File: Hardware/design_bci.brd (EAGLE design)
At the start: 53.3 x 59.7 mm, 13 parts, among them IC1 AD623N

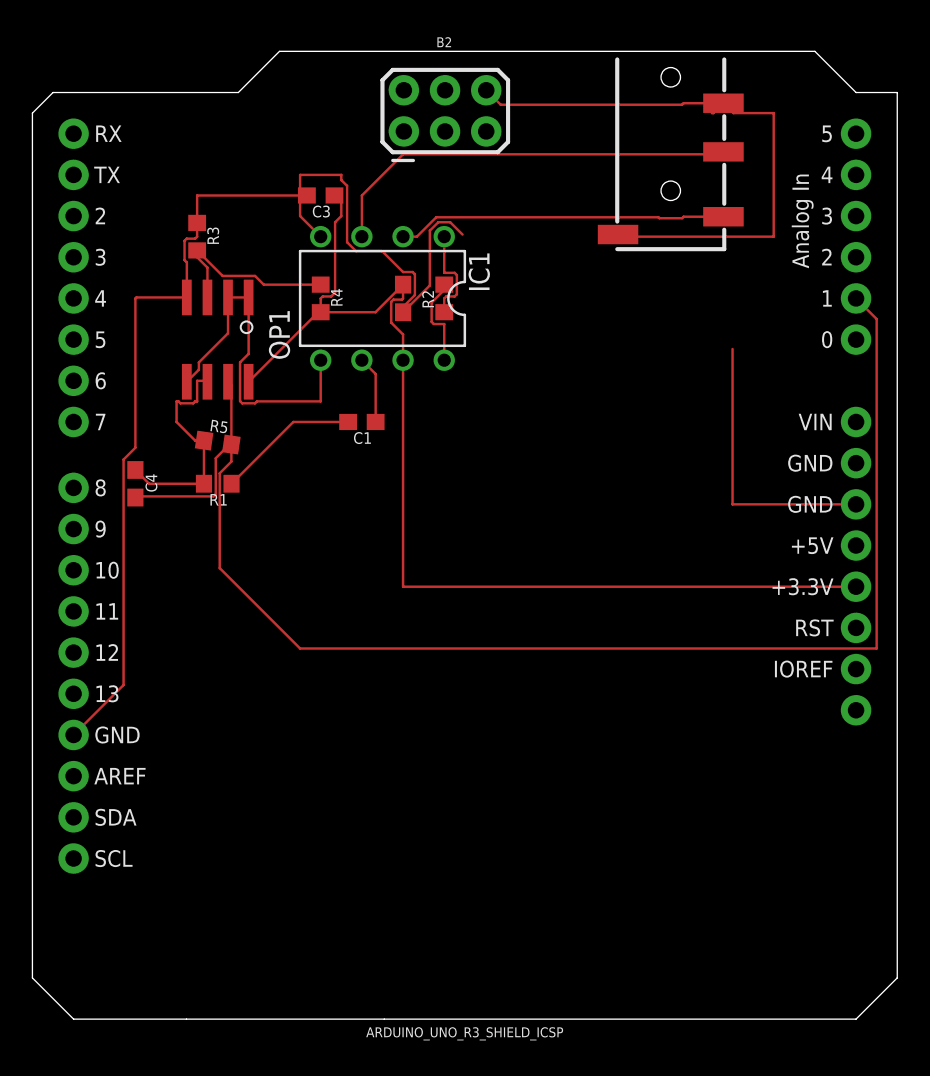
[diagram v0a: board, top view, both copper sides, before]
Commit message: updated
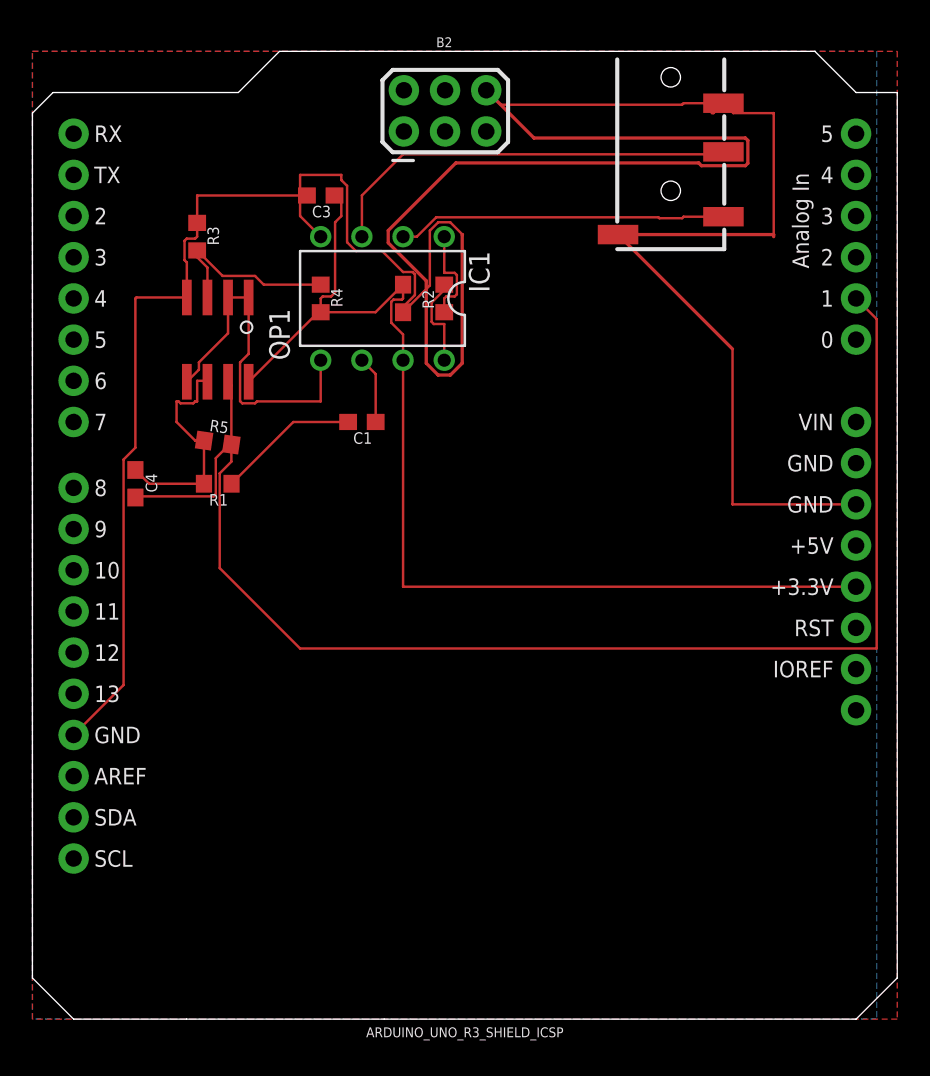
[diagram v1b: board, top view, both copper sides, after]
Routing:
- net GND: track 126.1 -> 199.1 mm
- added copper zone on layer 1, net 3.3V
- added copper zone on layer 16, net GND
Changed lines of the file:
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@@
 <wire x1="22.86" y1="43.6" x2="24.511" y2="45.251" width="0.1524" layer="1"/>
 <wire x1="24.511" y1="45.251" x2="24.511" y2="48.6282375" width="0.1524" layer="1"/>
-<wire x1="25.7682375" y1="49.149" x2="26.5272375" y2="48.39" width="0.1524" layer="1"/>
+<wire x1="26.5272375" y1="48.39" x2="25.7682375" y2="49.149" width="0.1524" layer="1"/>
 <wire x1="42.62" y1="56.49" x2="43.23" y2="55.88" width="0.1524" layer="1"/>
 <wire x1="43.23" y1="55.88" x2="45.72" y2="55.88" width="0.1524" layer="1"/>
-<wire x1="45.72" y1="55.88" x2="45.72" y2="48.26" width="0.1524" layer="1"/>
-<wire x1="45.72" y1="48.26" x2="36.25" y2="48.26" width="0.1524" layer="1"/>
+<wire x1="45.72" y1="48.26" x2="45.72" y2="55.88" width="0.1524" layer="1"/>
 <contactref element="B2" pad="GND@2"/>
 <contactref element="B2" pad="GND_ICSP"/>
@@
 <wire x1="41.91" y1="55.88" x2="41.91" y2="56.49" width="0.1524" layer="1"/>
 <contactref element="J1" pad="GND/MIC"/>
-<wire x1="36.12" y1="48.39" x2="36.25" y2="48.26" width="0" layer="19" extent="1-1"/>
-<wire x1="26.5272375" y1="48.39" x2="27.9900125" y2="57.29000625" width="0" layer="19" extent="1-1"/>
-<wire x1="43.18" y1="41.33" x2="36.25" y2="48.26" width="0" layer="19" extent="1-1"/>
+<wire x1="43.9752125" y1="54.344" x2="44.124" y2="54.1952125" width="0.2032" layer="1"/>
+<wire x1="44.124" y1="54.1952125" x2="44.124" y2="52.7847875" width="0.2032" layer="1"/>
+<wire x1="44.124" y1="52.7847875" x2="43.9752125" y2="52.636" width="0.2032" layer="1"/>
+<wire x1="43.9752125" y1="52.636" x2="41.2647875" y2="52.636" width="0.2032" layer="1"/>
+<wire x1="21.9456" y1="48.6387625" x2="21.9456" y2="47.8812375" width="0.2032" layer="1"/>
+<wire x1="25.0212375" y1="39.7256" x2="25.7787625" y2="39.7256" width="0.2032" layer="1"/>
+<wire x1="27.9900125" y1="57.29000625" x2="30.93601875" y2="54.344" width="0.2032" layer="1"/>
+<wire x1="41.2647875" y1="52.636" x2="41.0931875" y2="52.8076" width="0.2032" layer="1"/>
+<wire x1="30.93601875" y1="54.344" x2="43.9752125" y2="54.344" width="0.2032" layer="1"/>
+<wire x1="24.2912" y1="40.4556375" x2="25.0212375" y2="39.7256" width="0.2032" layer="1"/>
+<wire x1="41.0931875" y1="52.8076" x2="26.1144375" y2="52.8076" width="0.2032" layer="1"/>
+<wire x1="26.1144375" y1="52.8076" x2="21.9456" y2="48.6387625" width="0.2032" layer="1"/>
+<wire x1="24.2912" y1="45.5356375" x2="24.2912" y2="40.4556375" width="0.2032" layer="1"/>
+<wire x1="21.9456" y1="47.8812375" x2="24.2912" y2="45.5356375" width="0.2032" layer="1"/>
+<wire x1="26.5088" y1="48.3715625" x2="26.5272375" y2="48.39" width="0.2032" layer="1"/>
+<wire x1="25.7787625" y1="39.7256" x2="26.5088" y2="40.4556375" width="0.2032" layer="1"/>
+<wire x1="26.5088" y1="40.4556375" x2="26.5088" y2="48.3715625" width="0.2032" layer="1"/>
+<wire x1="36.12" y1="48.39" x2="43.18" y2="41.33" width="0.2032" layer="1"/>
+<polygon width="0.2032" layer="16">
+<vertex x="0" y="59.69"/>
+<vertex x="52.07" y="59.69"/>
+<vertex x="52.07" y="0"/>
+<vertex x="0" y="0"/>
+</polygon>
+<wire x1="36.12" y1="48.39" x2="45.72" y2="48.39" width="0.2032" layer="1"/>
+<wire x1="45.72" y1="48.39" x2="45.72" y2="48.26" width="0.2032" layer="1"/>
 </signal>
 <signal name="N$4">
@@
 <wire x1="19.05" y1="49.53" x2="19.05" y2="50.38" width="0.1524" layer="1"/>
 <wire x1="19.05" y1="50.38" x2="18.63" y2="50.8" width="0.1524" layer="1"/>
+<polygon width="0.2032" layer="1">
+<vertex x="0" y="59.69"/>
+<vertex x="53.34" y="59.69"/>
+<vertex x="53.34" y="0"/>
+<vertex x="0" y="0"/>
+</polygon>
 </signal>
 <signal name="N$9">
